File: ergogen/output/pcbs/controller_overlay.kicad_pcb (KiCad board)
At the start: 2 copper layers, 19.7 x 60.1 mm, 2 parts

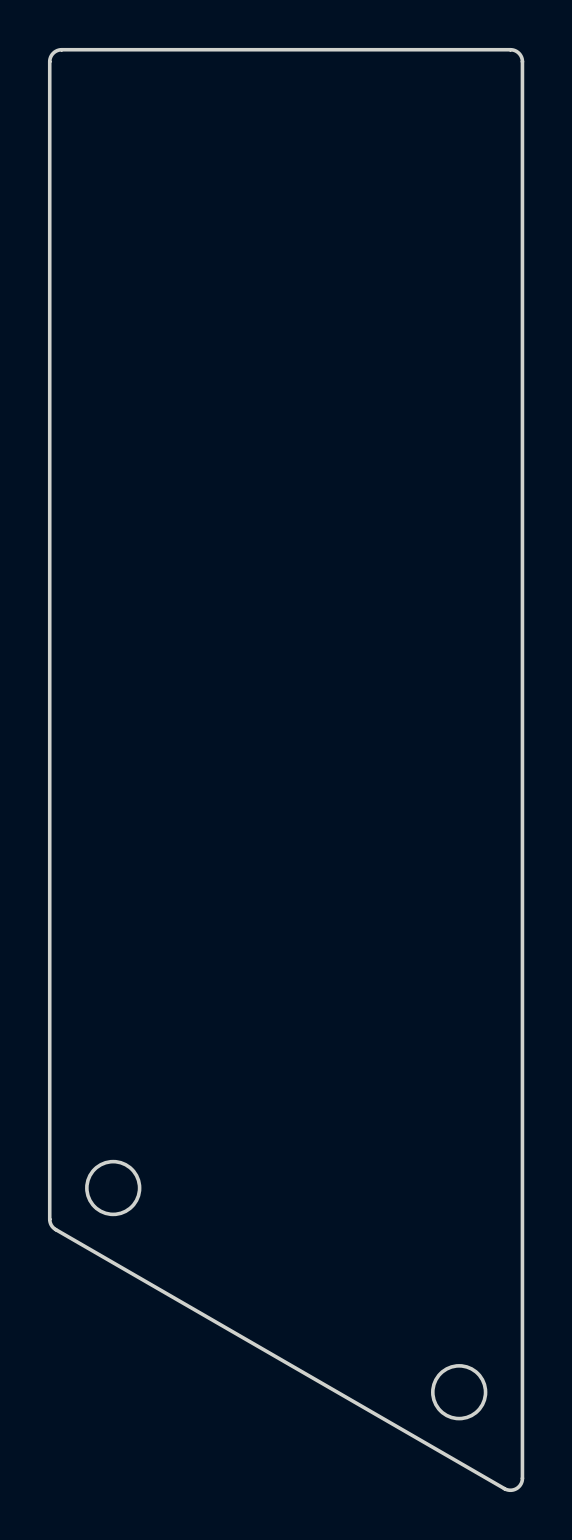
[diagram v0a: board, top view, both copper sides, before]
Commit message: Update assets
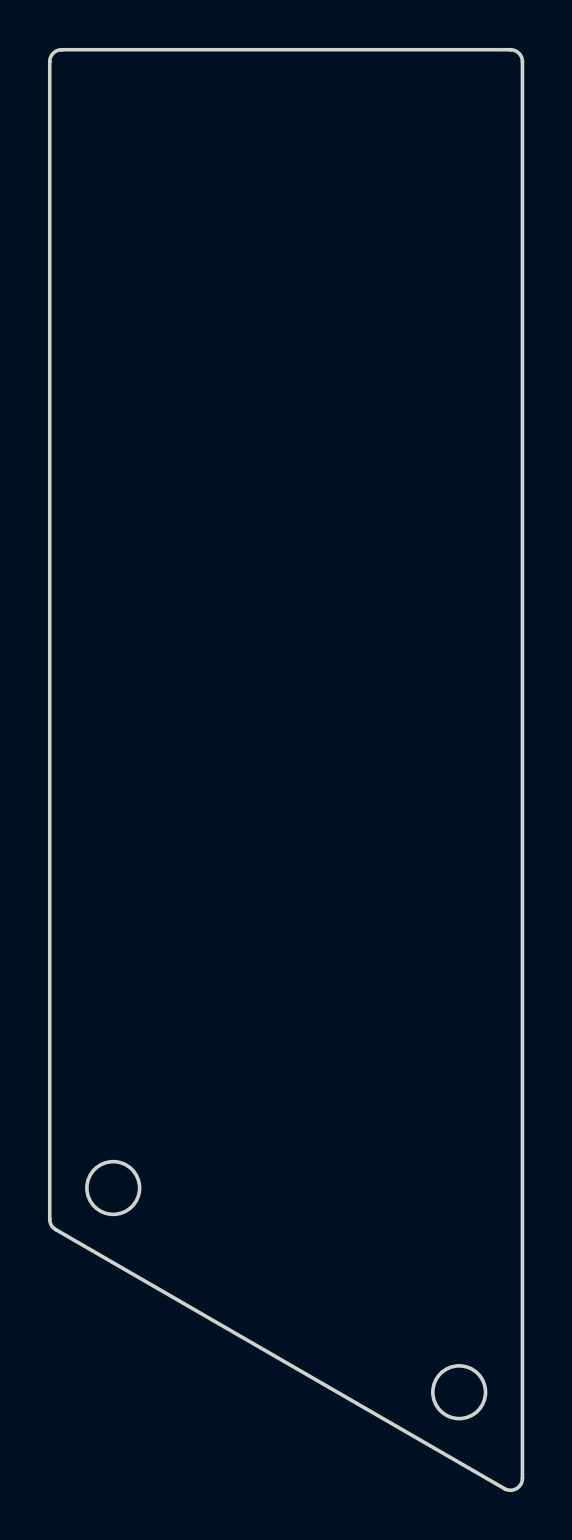
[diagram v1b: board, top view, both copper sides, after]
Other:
- net class Default removed
